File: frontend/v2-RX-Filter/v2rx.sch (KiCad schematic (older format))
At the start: 64 parts, among them P1 CONN_01X09, P4 CONN_01X02, P5 CONN_01X02, U1 4504, U10 PE4259-53, U11 PE4259-53, U12 PE4259-53, U2 PE4259-53, U3 PE4259-53, U4 PE4259-53, U5 PE4259-53, U6 PE4259-53, U7 PE4259-53, U8 PE4259-53, U9 PE4259-53

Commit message: new kicad 4.0.1 stable
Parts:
- C1, C10, C11, C12, C13, C14, C15, C16, C17, C18, C19, C2, C20, C21, C22, C23, C24, C25, C26, C3, C4, C5, C6, C7, C8, C9: symbol C -> C-RESCUE-v2rx
- P1: footprint (none) -> Socket_Strips:Socket_Strip_Straight_1x09
- U1: footprint (none) -> Housings_SOIC:SOIC-16_3.9x9.9mm_Pitch1.27mm
- U10, U11, U12, U2, U3, U4, U5, U6, U7, U8, U9: footprint (none) -> HERMESLITE:sc70-6

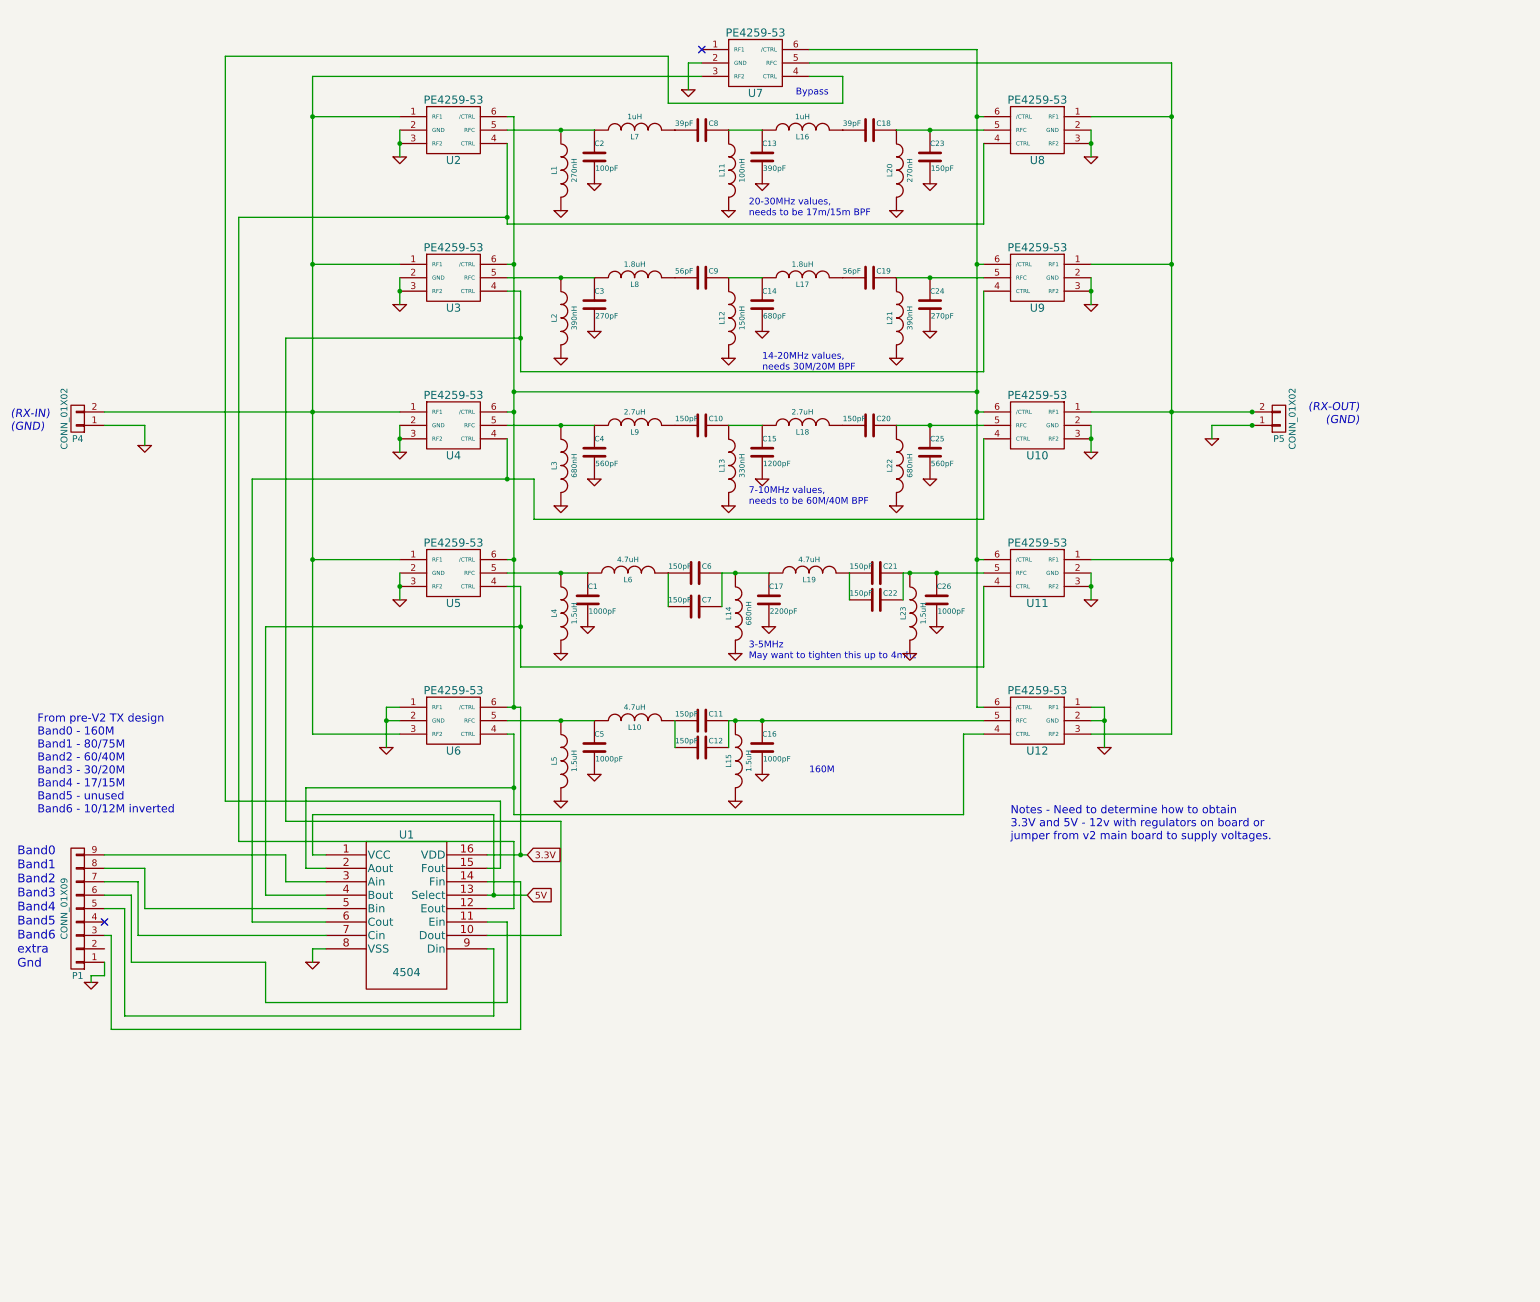
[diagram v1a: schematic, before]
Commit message: v2rx changes and update to new kicad
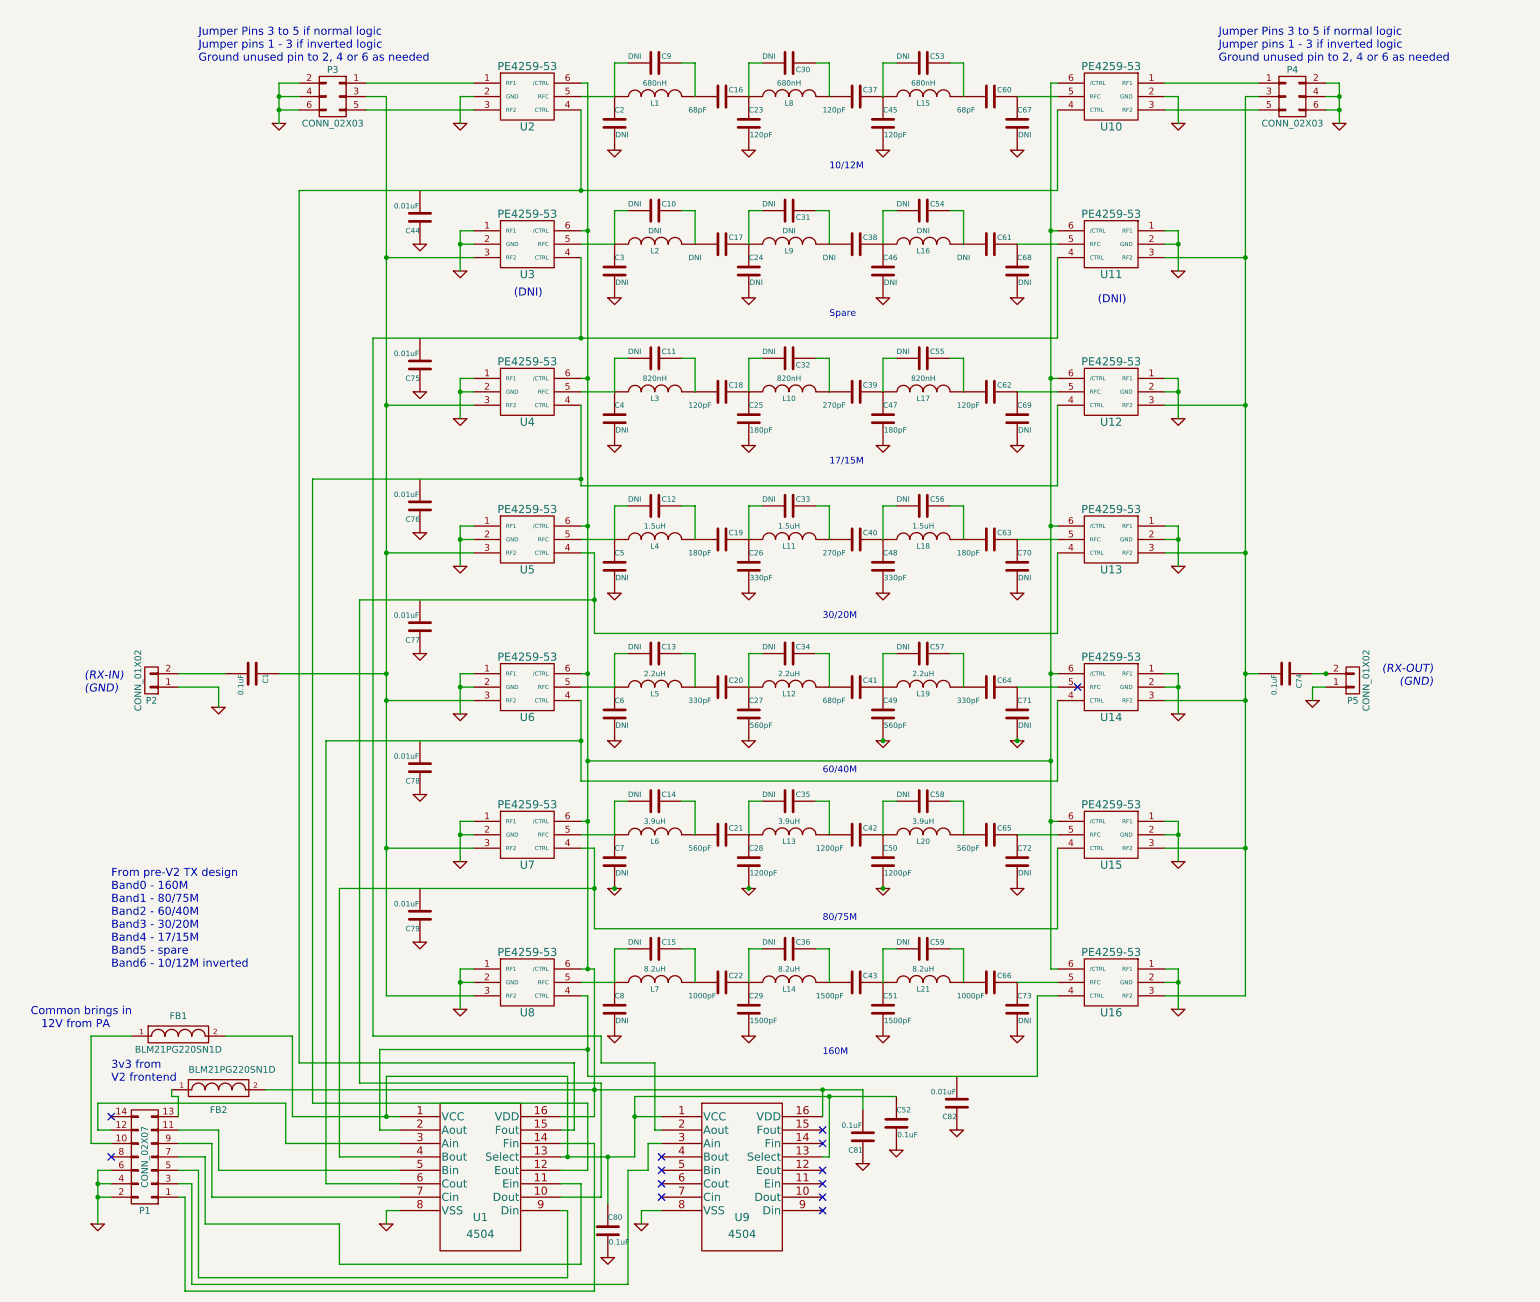
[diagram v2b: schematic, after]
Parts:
- removed C7: 150pF, HERMESLITE:C_0805, symbol C-RESCUE-v2rx
- removed L20: 270nH, HERMESLITE:Choke_SMD_1206_Standard, symbol INDUCTOR
- removed L22: 680nH, HERMESLITE:Choke_SMD_1206_Standard, symbol INDUCTOR
- removed L23: 1.5uH, HERMESLITE:Choke_SMD_1206_Standard, symbol INDUCTOR
- removed P1: CONN_01X09, Socket_Strips:Socket_Strip_Straight_1x09, symbol CONN_01X09
- removed U7: PE4259-53, HERMESLITE:sc70-6, symbol PE4259-53
- added C1, C52, C74, C80, C81: 0.1uF, HERMESLITE:C_0805, symbol C-RESCUE-v2rx
- added C17, C30, C31, C32, C33, C34, C35, C36, C38, C46, C53, C54, C55, C56, C57, C58, C59, C6, C61, C67, C68, C69, C70, C71, C73: DNI, HERMESLITE:C_0805, symbol C-RESCUE-v2rx
- added C26, C48, C64: 330pF, HERMESLITE:C_0805, symbol C-RESCUE-v2rx
- added C27, C49, C65: 560pF, HERMESLITE:C_0805, symbol C-RESCUE-v2rx
- added C29, C43, C51: 1500pF, HERMESLITE:C_0805, symbol C-RESCUE-v2rx
- added C37, C45, C62: 120pF, HERMESLITE:C_0805, symbol C-RESCUE-v2rx
- added C39, C40: 270pF, HERMESLITE:C_0805, symbol C-RESCUE-v2rx
- added C41: 680pF, HERMESLITE:C_0805, symbol C-RESCUE-v2rx
- added C44, C75, C76, C77, C78, C79, C82: 0.01uF, HERMESLITE:C_0805, symbol C-RESCUE-v2rx
- added C47, C63: 180pF, HERMESLITE:C_0805, symbol C-RESCUE-v2rx
- added C50: 1200pF, HERMESLITE:C_0805, symbol C-RESCUE-v2rx
- added C60: 68pF, HERMESLITE:C_0805, symbol C-RESCUE-v2rx
- added C66: 1000pF, HERMESLITE:C_0805, symbol C-RESCUE-v2rx
- added FB1, FB2: BLM21PG220SN1D, symbol FILTER
- added L19: 2.2uH, HERMESLITE:Choke_SMD_1206_Standard, symbol INDUCTOR
- added P1: CONN_02X07, symbol CONN_02X07
- added P3, P4: CONN_02X03, symbol CONN_02X03
- added U10, U11, U2, U3: PE4259-53, HERMESLITE:sc70-6, symbol PE4259-53
- added U9: 4504, Housings_SOIC:SOIC-16_3.9x9.9mm_Pitch1.27mm, symbol 4504
- C10, C11, C12: value 150pF -> DNI
- C13: value 390pF -> DNI
- C14: value 680pF -> DNI
- C15: value 1200pF -> DNI
- C16: value 1000pF -> 68pF
- C18: value 39pF -> 120pF
- C19: value 56pF -> 180pF
- C2: value 100pF -> DNI
- C20: value 150pF -> 330pF
- C21: renamed from C6; value 150pF -> 560pF
- C22: value 150pF -> 1000pF
- C23: value 150pF -> 120pF
- C24, C3: value 270pF -> DNI
- C25: value 560pF -> 180pF
- C28: renamed from C17; value 2200pF -> 1200pF
- C4: value 560pF -> DNI
- C42: renamed from C21; value 150pF -> 1200pF
- C5: value 1000pF -> DNI
- C7: renamed from C1; value 1000pF -> DNI
- C72: renamed from C26; value 1000pF -> DNI
- C8: value 39pF -> DNI
- C9: value 56pF -> DNI
- L1: value 270nH -> 680nH
- L10: value 4.7uH -> 820nH
- L11: value 100nH -> 1.5uH
- L12: value 150nH -> 2.2uH
- L13: value 330nH -> 3.9uH
- L14: value 680nH -> 8.2uH
- L15: value 1.5uH -> 680nH
- L16: value 1uH -> DNI
- L17: value 1.8uH -> 820nH
- L18: value 2.7uH -> 1.5uH
- L2: value 390nH -> DNI
- L20: renamed from L19; value 4.7uH -> 3.9uH
- L21: value 390nH -> 8.2uH
- L3: value 680nH -> 820nH
- L5: value 1.5uH -> 2.2uH
- L6: value 4.7uH -> 3.9uH
- L7: value 1uH -> 8.2uH
- L8: value 1.8uH -> 680nH
- L9: value 2.7uH -> DNI
- renumbered P4 to P2, U8 to U12, U9 to U13, U10 to U14, U11 to U15, U12 to U16, U2 to U4, U3 to U5, U4 to U6, U5 to U7, U6 to U8
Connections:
- net GND: now also C8.2, U12.1 (RF1), U13.1 (RF1), U14.1 (RF1), U15.1 (RF1), U4.1 (RF1), U5.1 (RF1), U6.1 (RF1), U7.1 (RF1), C26.2, C27.2, C29.2, C44.1, C45.2, C46.2, C47.2, C48.2, C49.2, C50.2, C51.2, C52.2, C6.2, C67.2, C68.2, C69.2, C70.2, C71.2, C73.2, C75.1, C76.1, C77.1, C78.1, C79.1, C80.2, C81.1, C82.1, P1.2 (P2), P1.4 (P4), P1.6 (P6), P3.2 (P2), P3.4 (P4), P3.6 (P6), P4.2 (P2), P4.4 (P4), P4.6 (P6), U10.2 (GND), U11.1 (RF1), U11.2 (GND), U2.2 (GND), U3.1 (RF1), U3.2 (GND), U9.8 (VSS); no longer C13.2, C14.2, C15.2, C16.2, L1.2, L11.2, L12.2, L13.2, L14.2, L15.2, L2.2, L21.2, L3.2, L4.2, L5.2, U12.3 (RF2), U13.3 (RF2), U14.3 (RF2), U15.3 (RF2), U4.3 (RF2), U5.3 (RF2), U6.3 (RF2), U7.3 (RF2)
- net at C2.1, L1.1: now also C9.2, U2.5 (RFC); no longer L7.1, U4.5 (RFC)
- net at L7.2: now also C15.1, C22.2; no longer C8.2
- net at C18.2: now also C11.1, L3.2; no longer L16.2
- net at C4.1, L3.1: now also C11.2, U4.5 (RFC); no longer L9.1, U6.5 (RFC)
- net at C10.2: now also C3.1, L2.1, U3.5 (RFC); no longer L9.2
- net at C20.2: now also C13.1, L5.2; no longer L18.2
- net at L8.2: now also C30.1, C37.2; no longer C9.2
- net at C19.2: now also C12.1, L4.2; no longer L17.2
- net at C7.1, L6.1, U7.5 (RFC): now also C14.2; no longer L4.1
- net at C21.1, C28.1: now also L13.1, C35.2; no longer L14.1, L20.1
- net at C21.2, L6.2: now also C14.1
- net at C72.1, U15.5 (RFC): now also C65.1; no longer C22.1, C42.1
- net at U1.14 (Fin): now also P1.1 (P1)
- net at U1.9 (Din): now also P1.5 (P5)
- net at U1.11 (Ein): now also P1.7 (P7)
- net at U1.7 (Cin): now also P1.9 (P9)
- net at U1.5 (Bin): now also P1.11 (P11)
- net at U1.3 (Ain): now also P1.12 (P12)
- net at U1.15 (Fout): now also U10.4 (CTRL), U2.4 (CTRL)
- net 3.3V: no longer names the net of U1.16 (VDD), U12.6 (/CTRL), U13.6 (/CTRL), U14.6 (/CTRL), U15.6 (/CTRL), U16.6 (/CTRL), U4.6 (/CTRL), U5.6 (/CTRL), U6.6 (/CTRL), U7.6 (/CTRL), U8.6 (/CTRL)
- net 3.3V: now also C81.2, FB2.2, U10.6 (/CTRL), U11.6 (/CTRL), U2.6 (/CTRL), U3.6 (/CTRL), U9.16 (VDD)
- net 5V: no longer names the net of U1.1 (VCC), U1.13 (Select)
- net 5V: now also C52.1, C80.1, FB1.2, U9.1 (VCC), U9.13 (Select)
- new net: C74.1, P5.2 (P2)
- new net: C1.2, P2.2 (P2)
- new net: C42.1, C50.1, C58.2, L20.1
- new net: C35.1, C42.2, L13.2
- new net: C58.1, C65.2, L20.2
- new net: C1.1, P3.3 (P3), U3.3 (RF2), U4.3 (RF2), U5.3 (RF2), U6.3 (RF2), U7.3 (RF2), U8.3 (RF2)
- new net: C15.2, C8.1, L7.1, U8.5 (RFC)
- new net: C74.2, P4.3 (P3), U11.3 (RF2), U12.3 (RF2), U13.3 (RF2), U14.3 (RF2), U15.3 (RF2), U16.3 (RF2)
- new net: C66.1, C73.1, U16.5 (RFC)
- new net: C13.2, C6.1, L5.1, U6.5 (RFC)
- new net: C12.2, C5.1, L4.1, U5.5 (RFC)
- new net: C64.1, C71.1, U14.5 (RFC)
- new net: C63.1, C70.1, U13.5 (RFC)
- new net: C62.1, C69.1, U12.5 (RFC)
- new net: FB1.1, P1.10 (P10)
- new net: FB2.1, P1.13 (P13)
- new net: P1.3 (P3), U9.3 (Ain)
- new net: C22.1, C29.1, C36.2, L14.1
- new net: C43.1, C51.1, C59.2, L21.1
- new net: C36.1, C43.2, L14.2
- new net: C59.1, C66.2, L21.2
- new net: C20.1, C27.1, C34.2, L12.1
- new net: C41.1, C49.1, C57.2, L19.1
- new net: C34.1, C41.2, L12.2
- new net: C57.1, C64.2, L19.2
- new net: C19.1, C26.1, C33.2, L11.1
- new net: C40.1, C48.1, C56.2, L18.1
- new net: C33.1, C40.2, L11.2
- new net: C56.1, C63.2, L18.2
- new net: C18.1, C25.1, C32.2, L10.1
- new net: C39.1, C47.1, C55.2, L17.1
- new net: C32.1, C39.2, L10.2
- new net: C55.1, C62.2, L17.2
- new net: U11.4 (CTRL), U3.4 (CTRL), U9.2 (Aout)
- new net: C61.1, C68.1, U11.5 (RFC)
- new net: C17.1, C24.1, C31.2, L9.1
- new net: C10.1, C17.2, L2.2
- new net: C38.1, C46.1, C54.2, L16.1
- new net: C31.1, C38.2, L9.2
- new net: C54.1, C61.2, L16.2
- new net: P3.1 (P1), U2.1 (RF1)
- new net: P3.5 (P5), U2.3 (RF2)
- new net: P4.1 (P1), U10.1 (RF1)
- new net: P4.5 (P5), U10.3 (RF2)
- new net: C60.1, C67.1, U10.5 (RFC)
- new net: C16.1, C23.1, C30.2, L8.1
- new net: C16.2, C9.1, L1.2
- new net: C37.1, C45.1, C53.2, L15.1
- new net: C53.1, C60.2, L15.2
- no-connect marks 2 -> 13
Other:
- note added: "(DNI)"
- note added: "10/12M\n"
- note added: "160M\n"
- note added: "17/15M\n"
- note added: "30/20M\n"
- note added: "3v3 from\nV2 frontend"
- note added: "60/40M\n"
- note added: "80/75M\n"
- note added: "Common brings in\n 12V from PA"
- note added: "From pre-V2 TX design\nBand0 - 160M\nBand1 - 80/75M\nBand2 - 60/40M\nBand3 - 30/20M\nBand4 - 17/15M\nBand5 - spare\nBand6 - 10/12M inverted"
- note added: "Jumper Pins 3 to 5 if normal logic\nJumper pins 1 - 3 if inverted logic\nGround unused pin to 2, 4 or 6 as needed"
- note added: "Spare\n"
- note removed: "14-20MHz values,\nneeds 30M/20M BPF"
- note removed: "160M"
- note removed: "20-30MHz values,\nneeds to be 17m/15m BPF"
- note removed: "3-5MHz\nMay want to tighten this up to 4mhz"
- note removed: "7-10MHz values,\nneeds to be 60M/40M BPF"
- note removed: "Band0\nBand1\nBand2\nBand3\nBand4\nBand5\nBand6\nextra\nGnd"
- note removed: "Bypass"
- note removed: "From pre-V2 TX design\nBand0 - 160M\nBand1 - 80/75M\nBand2 - 60/40M\nBand3 - 30/20M\nBand4 - 17/15M\nBand5 - unused\nBand6 - 10/12M inverted"
- note removed: "Notes - Need to determine how to obtain\n3.3V and 5V - 12v with regulators on board or\njumper from v2 main board to supply voltages."
- moved on the sheet: C21, C28, C42, C7, C72, L20, L6, P2, P5, U1, U12, U13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
